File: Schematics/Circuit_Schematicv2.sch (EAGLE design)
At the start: 66 parts, among them Q2 LE33CZ

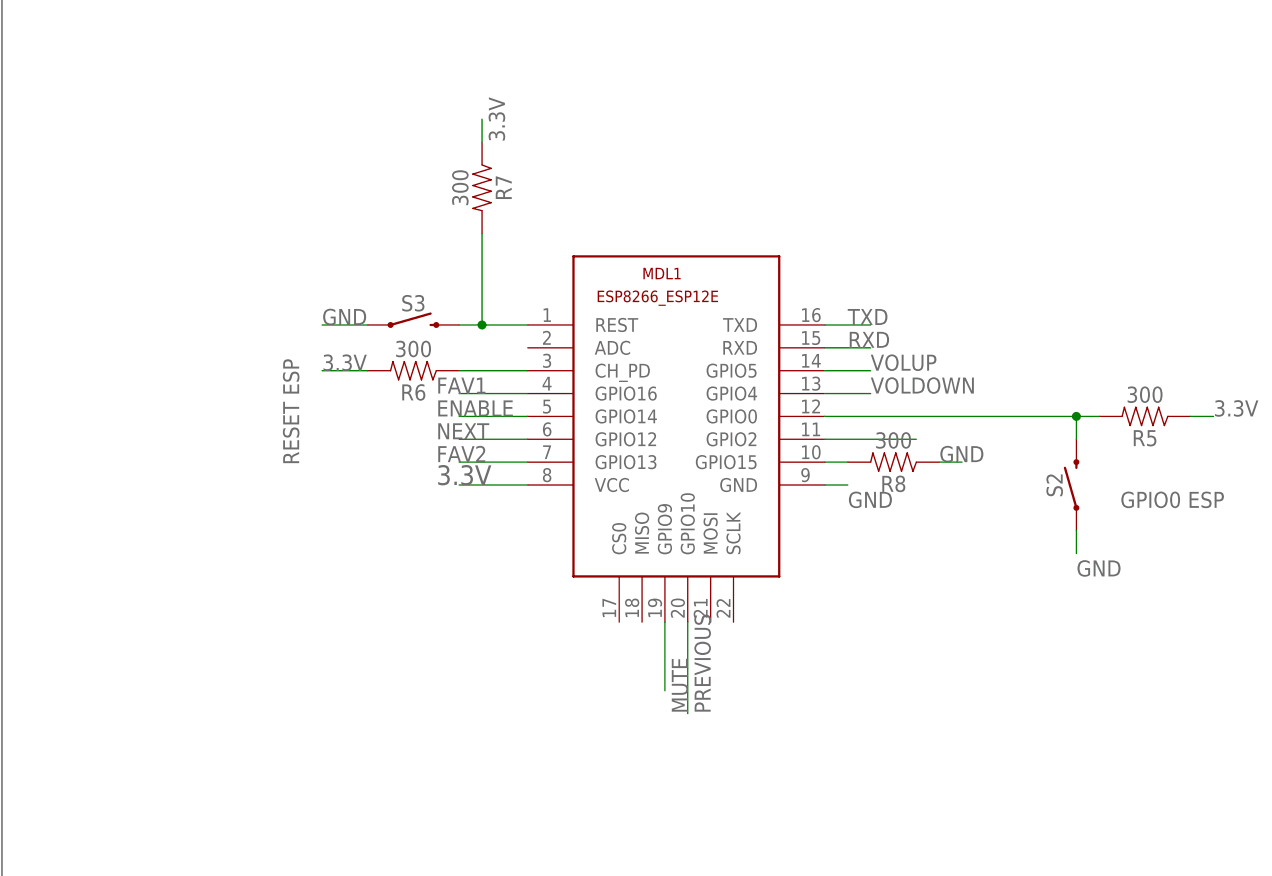
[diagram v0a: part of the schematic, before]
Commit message: Final changes to make ESP work
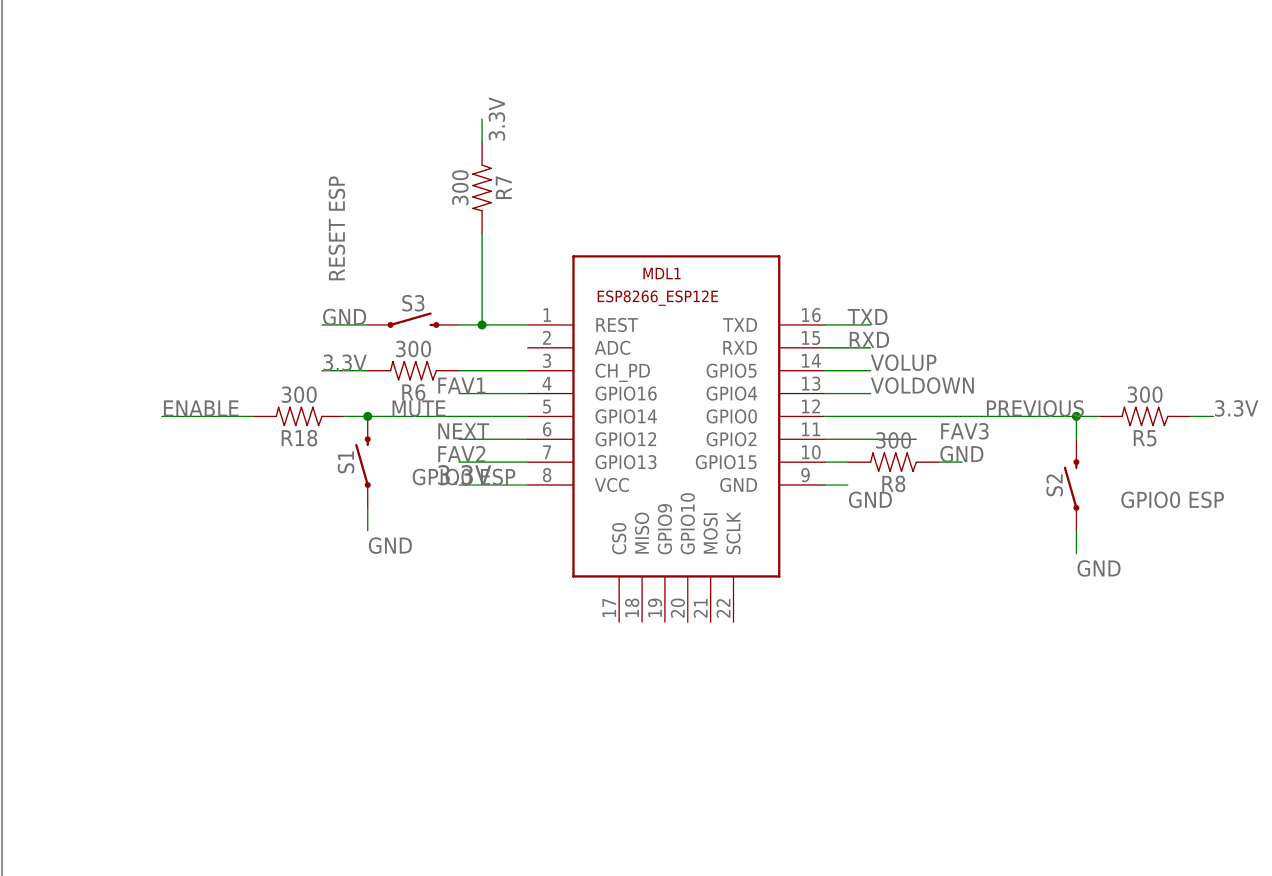
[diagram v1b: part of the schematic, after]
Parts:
- added R18: 300, SparkFun-Resistors:1OHM-0603-1/10W-1%
- added S1: GPIO0 ESP, SparkFun-Switches:MOMENTARY-SWITCH-SPST-SMD-6.0X3.5MM
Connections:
- removed net N$8: MDL1.GPIO0, R5.2, S2.2
- net ENABLE: now also R18.2; no longer MDL1.GPIO14
- net GND: now also S1.1
- net MUTE: now also MDL1.GPIO14, R18.1, S1.2; no longer MDL1.GPIO9
- net PREVIOUS: now also MDL1.GPIO0, R5.2, S2.2; no longer MDL1.GPIO10
